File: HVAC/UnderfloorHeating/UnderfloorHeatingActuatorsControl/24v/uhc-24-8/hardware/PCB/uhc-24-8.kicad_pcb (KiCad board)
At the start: 2 copper layers, 118.1 x 69.8 mm, 57 parts, among them J1 WJ126V-5.0-2P, J10 WJ126V-5.0-2P, J11 WJ126V-5.0-2P, J2 ESP-PROG, J3 Conn_02x06_Counter_Clockwise, J4 WJ126V-5.0-2P, J5 WJ126V-5.0-2P, J6 WJ126V-5.0-2P, J7 WJ126V-5.0-2P, J8 WJ126V-5.0-2P, J9 WJ126V-5.0-2P, Q1 2N7002P, Q2 2N7002P, Q3 2N7002P, Q4 2N7002P, Q5 2N7002P, Q6 2N7002P, Q7 2N7002P, Q8 2N7002P, U1 ESP32-WROOM-32D, U2 LM3671MFX-3.3/NOPB

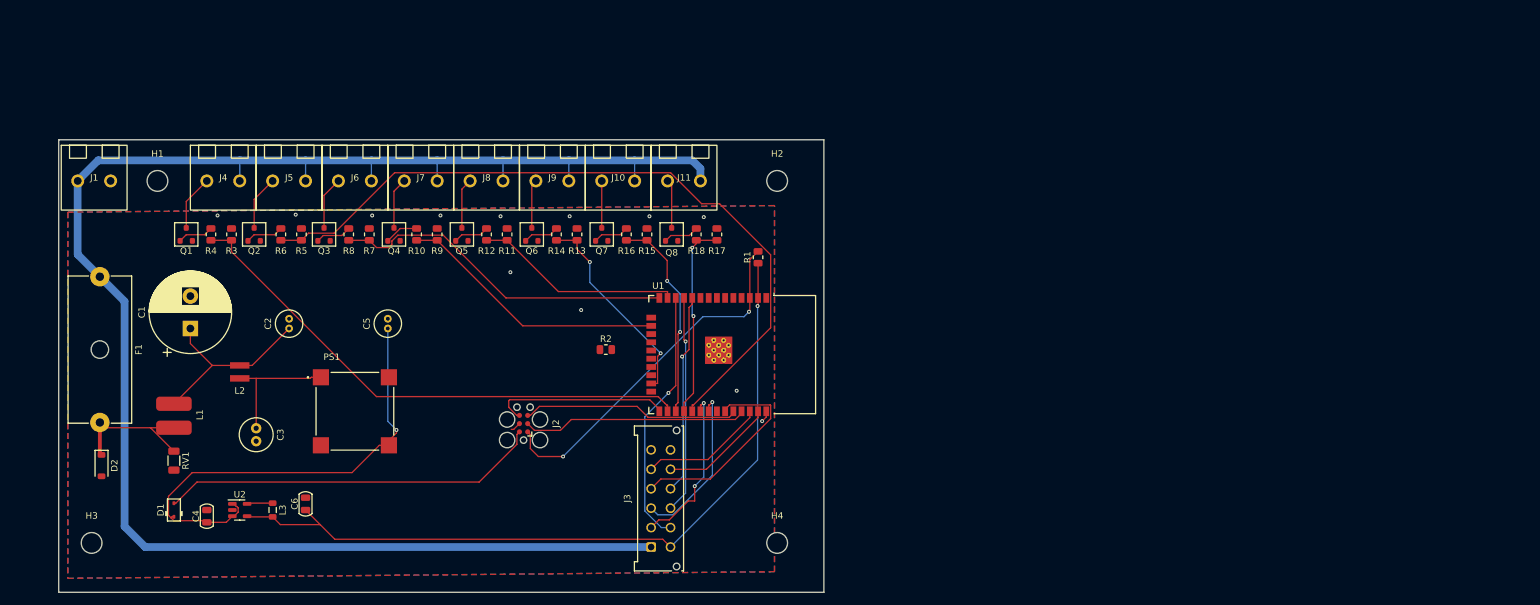
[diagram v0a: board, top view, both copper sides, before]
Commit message: Ready for fabrication
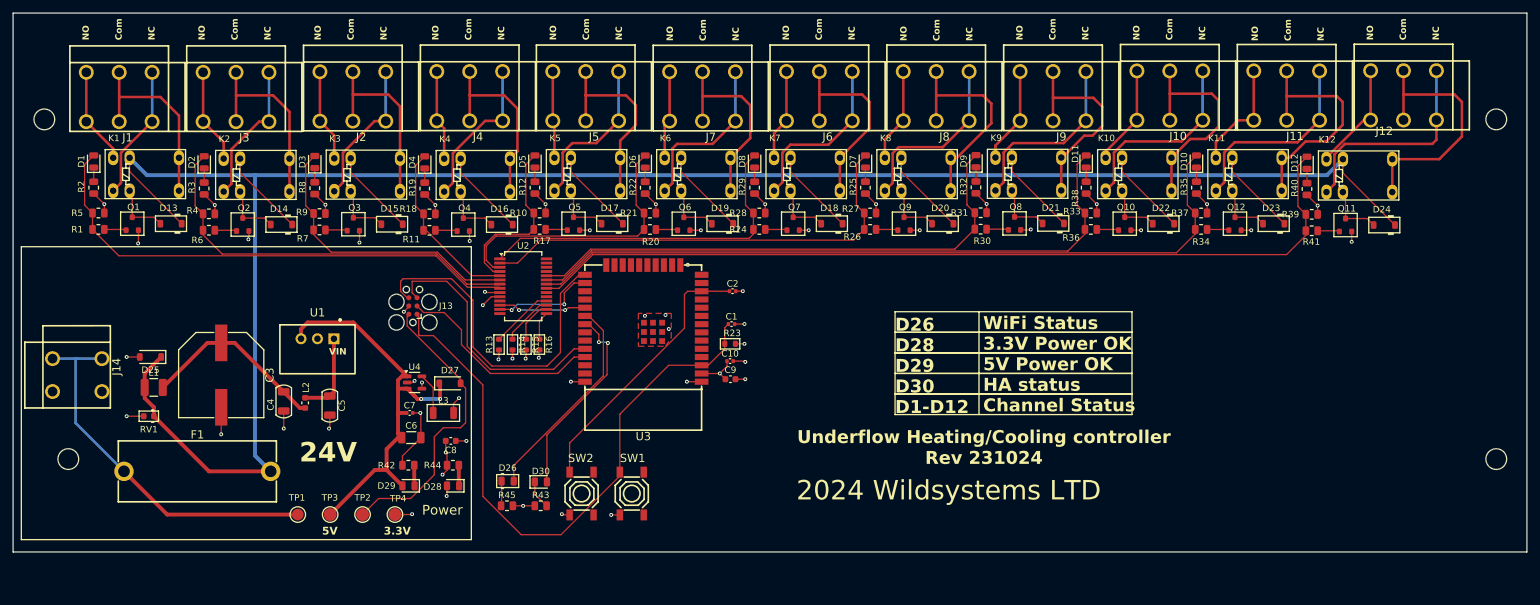
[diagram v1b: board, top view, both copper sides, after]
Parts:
- removed PS1: K7805JT-500R3-LB, K7805JT-500R3:CONV_K7805JT-500R3-LB
- added C10: 0.1uF, Capacitor_SMD:C_0402_1005Metric, F.Cu at (141.7, 91.3)
- added C7: 4.7uF/10V, Capacitor_SMD:C_0402_1005Metric, F.Cu at (92.3, 99.3)
- added C8: 10uF, Capacitor_SMD:C_0603_1608Metric, F.Cu at (98.6, 103.6)
- added C9: 22uF, Capacitor_SMD:C_0603_1608Metric, F.Cu at (141.8, 94.1)
- added D10: KT-0805Y, LED_SMD:LED_0805_2012Metric, F.Cu at (213.7, 60.5)
- added D11: KT-0805Y, LED_SMD:LED_0805_2012Metric, F.Cu at (196.7, 60.5)
- added D12: KT-0805Y, LED_SMD:LED_0805_2012Metric, F.Cu at (230.8, 60.7)
- added D13: 1N4148W, PCM_Diode_SMD_AKL:D_SOD-123, F.Cu at (55.4, 70.1)
- added D14: 1N4148W, PCM_Diode_SMD_AKL:D_SOD-123, F.Cu at (72.5, 70.2)
- added D15: 1N4148W, PCM_Diode_SMD_AKL:D_SOD-123, F.Cu at (89.6, 70.2)
- added D16: 1N4148W, PCM_Diode_SMD_AKL:D_SOD-123, F.Cu at (106.5, 70.2)
- added D17: 1N4148W, PCM_Diode_SMD_AKL:D_SOD-123, F.Cu at (123.5, 70.1)
- added D18: 1N4148W, PCM_Diode_SMD_AKL:D_SOD-123, F.Cu at (157.4, 70.1)
- added D19: 1N4148W, PCM_Diode_SMD_AKL:D_SOD-123, F.Cu at (140.6, 70.1)
- added D20: 1N4148W, PCM_Diode_SMD_AKL:D_SOD-123, F.Cu at (174.6, 70.1)
- added D21: 1N4148W, PCM_Diode_SMD_AKL:D_SOD-123, F.Cu at (191.6, 70.1)
- added D22: 1N4148W, PCM_Diode_SMD_AKL:D_SOD-123, F.Cu at (208.6, 70.1)
- added D23: 1N4148W, PCM_Diode_SMD_AKL:D_SOD-123, F.Cu at (225.6, 70.1)
- added D24: 1N4148W, PCM_Diode_SMD_AKL:D_SOD-123, F.Cu at (242.7, 70.3)
- added D25: BAT46W, Diode_SMD:D_SOD-123, F.Cu at (52.3, 90.7)
- added D26: KT-0805B, Diode_SMD_AKL:D_0805_2012Metric, F.Cu at (107.4, 109.8)
- added D27: 1N5819, Diode_SMD:D_SOD-123, F.Cu at (98.5, 94.7)
- added D28: KT-0805G, LED_SMD:LED_0805_2012Metric, F.Cu at (99.0, 110.6)
- added D29: KT-0805G, LED_SMD:LED_0805_2012Metric, F.Cu at (92.1, 110.6)
- added D3: KT-0805Y, LED_SMD:LED_0805_2012Metric, F.Cu at (77.6, 60.6)
- added D30: KT-0805G, LED_SMD:LED_0805_2012Metric, F.Cu at (112.5, 110.0)
- added D4: KT-0805Y, LED_SMD:LED_0805_2012Metric, F.Cu at (94.6, 60.6)
- added D5: KT-0805Y, LED_SMD:LED_0805_2012Metric, F.Cu at (111.6, 60.5)
- added D6: KT-0805Y, LED_SMD:LED_0805_2012Metric, F.Cu at (128.6, 60.5)
- added D7: KT-0805Y, LED_SMD:LED_0805_2012Metric, F.Cu at (162.6, 60.5)
- added D8: KT-0805Y, LED_SMD:LED_0805_2012Metric, F.Cu at (145.5, 60.5)
- added D9: KT-0805Y, LED_SMD:LED_0805_2012Metric, F.Cu at (179.7, 60.5)
- added J12: WJ126V-5.0-3P, My Footprints:CONN-TH_3P-P5.08_DIBO_DB142V-5.08-3P, F.Cu at (245.7, 50.3)
- added J13: ESP-PROG, Connector:Tag-Connect_TC2030-IDC-FP_2x03_P1.27mm_Vertical, F.Cu at (92.8, 82.8)
- added J14: WJ126V-5.0-2P, My Footprints:CONN-TH_2P-P5.08_DIBO_DB142V-5.08-2P, F.Cu at (41.0, 93.5)
- added K1: BSC-SS-124L, My Footprints:Relay_SPDT_QLRELAY_BSC, F.Cu at (56.7, 59.9)
- added K10: BSC-SS-124L, My Footprints:Relay_SPDT_QLRELAY_BSC, F.Cu at (209.9, 59.9)
- added K11: BSC-SS-124L, My Footprints:Relay_SPDT_QLRELAY_BSC, F.Cu at (226.9, 59.9)
- added K12: BSC-SS-124L, My Footprints:Relay_SPDT_QLRELAY_BSC, F.Cu at (244.0, 60.1)
- added K2: BSC-SS-124L, My Footprints:Relay_SPDT_QLRELAY_BSC, F.Cu at (73.7, 60.1)
- added K3: BSC-SS-124L, My Footprints:Relay_SPDT_QLRELAY_BSC, F.Cu at (90.8, 60.0)
- added K4: BSC-SS-124L, My Footprints:Relay_SPDT_QLRELAY_BSC, F.Cu at (107.8, 60.1)
- added K5: BSC-SS-124L, My Footprints:Relay_SPDT_QLRELAY_BSC, F.Cu at (124.8, 59.9)
- added K6: BSC-SS-124L, My Footprints:Relay_SPDT_QLRELAY_BSC, F.Cu at (141.8, 59.9)
- added K7: BSC-SS-124L, My Footprints:Relay_SPDT_QLRELAY_BSC, F.Cu at (158.7, 59.9)
- added K8: BSC-SS-124L, My Footprints:Relay_SPDT_QLRELAY_BSC, F.Cu at (175.8, 59.9)
- added K9: BSC-SS-124L, My Footprints:Relay_SPDT_QLRELAY_BSC, F.Cu at (192.9, 59.9)
- added Q10: 2N7002P, Package_TO_SOT_SMD_AKL:SOT-23, F.Cu at (202.7, 70.1)
- added Q11: 2N7002P, Package_TO_SOT_SMD_AKL:SOT-23, F.Cu at (236.7, 70.3)
- added Q12: 2N7002P, Package_TO_SOT_SMD_AKL:SOT-23, F.Cu at (219.7, 70.1)
- added Q9: 2N7002P, Package_TO_SOT_SMD_AKL:SOT-23, F.Cu at (168.6, 70.1)
- added R19: 56R, Resistor_SMD:R_0805_2012Metric, F.Cu at (94.6, 64.7)
- added R20: 510R, Resistor_SMD:R_0805_2012Metric, F.Cu at (129.4, 71.0)
- added R21: 4.7k, Resistor_SMD:R_0805_2012Metric, F.Cu at (129.4, 68.5)
- added R22: 56R, Resistor_SMD:R_0805_2012Metric, F.Cu at (128.6, 64.5)
- added R23: 10K, PCM_Resistor_SMD_AKL:R_0603_1608Metric, F.Cu at (141.7, 88.6)
- added R24: 510R, Resistor_SMD:R_0805_2012Metric, F.Cu at (146.2, 71.0)
- added R25: 56R, Resistor_SMD:R_0805_2012Metric, F.Cu at (162.6, 64.5)
- added R26: 510R, Resistor_SMD:R_0805_2012Metric, F.Cu at (163.4, 71.0)
- added R27: 4.7k, Resistor_SMD:R_0805_2012Metric, F.Cu at (163.4, 68.5)
- added R28: 4.7k, Resistor_SMD:R_0805_2012Metric, F.Cu at (146.2, 68.5)
- added R29: 56R, Resistor_SMD:R_0805_2012Metric, F.Cu at (145.5, 64.5)
- added R30: 510R, Resistor_SMD:R_0805_2012Metric, F.Cu at (180.4, 70.9)
- added R31: 4.7k, Resistor_SMD:R_0805_2012Metric, F.Cu at (180.4, 68.4)
- added R32: 56R, Resistor_SMD:R_0805_2012Metric, F.Cu at (179.7, 64.5)
- added R33: 4.7k, Resistor_SMD:R_0805_2012Metric, F.Cu at (197.4, 68.5)
- added R34: 510R, Resistor_SMD:R_0805_2012Metric, F.Cu at (214.4, 71.0)
- added R35: 56R, Resistor_SMD:R_0805_2012Metric, F.Cu at (213.7, 64.5)
- added R36: 510R, Resistor_SMD:R_0805_2012Metric, F.Cu at (197.4, 71.0)
- added R37: 4.7k, Resistor_SMD:R_0805_2012Metric, F.Cu at (214.4, 68.5)
- added R38: 56R, Resistor_SMD:R_0805_2012Metric, F.Cu at (196.7, 64.5)
- added R39: 4.7k, Resistor_SMD:R_0805_2012Metric, F.Cu at (231.5, 68.7)
- added R40: 56R, Resistor_SMD:R_0805_2012Metric, F.Cu at (230.8, 64.7)
- added R41: 510R, Resistor_SMD:R_0805_2012Metric, F.Cu at (231.5, 71.2)
- added R42: 20R, Resistor_SMD:R_0805_2012Metric, F.Cu at (92.1, 107.4)
- added R43: 20R, Resistor_SMD:R_0805_2012Metric, F.Cu at (112.5, 113.6)
- added R44: 20R, Resistor_SMD:R_0805_2012Metric, F.Cu at (98.9, 107.4)
- added R45: 15R, Resistor_SMD:R_0805_2012Metric, F.Cu at (107.3, 113.6)
- added SW1: Reboot, My Footprints:SW-SMD_4P-L5.1-W5.1-P3.70-LS6.5-TL-2, F.Cu at (126.6, 111.8)
- added SW2: Clear, My Footprints:SW-SMD_4P-L5.1-W5.1-P3.70-LS6.5-TL-2, F.Cu at (118.8, 111.8)
- added TP1: 24V, TestPoint:TestPoint_Pad_D2.0mm, F.Cu at (75.0, 115.0)
- added TP2: 5V_USB, TestPoint:TestPoint_Pad_D2.0mm, F.Cu at (85.0, 115.0)
- added TP3: 5V, TestPoint:TestPoint_Pad_D2.0mm, F.Cu at (80.0, 115.0)
- added TP4: 3.3V, TestPoint:TestPoint_Pad_D2.0mm, F.Cu at (90.0, 115.0)
- added U3: ESP32-WROOM-32D, My Footprints:WIFI-SMD_ESP32-WROOM-32E-A, F.Cu at (128.3, 85.5)
- added U4: LM3671MFX-3.3/NOPB, Package_TO_SOT_SMD:TSOT-23-5, F.Cu at (93.0, 94.6)
- C1: value 680uF/50V -> 1uF; footprint Capacitor_THT:CP_Radial_D12.5mm_P5.00mm -> Capacitor_SMD:C_0402_1005Metric
- C2: value 4.7uF/50V -> 0.1uF; footprint Capacitor_THT_AKL:C_Radial_D4.0mm_H5.0mm_P1.50mm -> Capacitor_SMD:C_0402_1005Metric
- C3: value 10uF/50V -> 680uF/50V; footprint Capacitor_THT:C_Radial_D5.0mm_H11.0mm_P2.00mm -> My Footprints:CAP-SMD_BD12.5-L13.0-W13.0-LS14.4-FD
- C4: value 4.7uF -> 4.7uF/63V; footprint Capacitor_SMD_AKL:C_0805_2012Metric -> Capacitor_SMD_AKL:C_1206_3216Metric
- C5: value 22uF/10V -> 10uF/50V; footprint Capacitor_THT:C_Radial_D4.0mm_H7.0mm_P1.50mm -> Capacitor_SMD_AKL:C_1206_3216Metric
- C6: value 10uF -> 22uF/10V; footprint Capacitor_SMD_AKL:C_0805_2012Metric -> Capacitor_SMD:C_1206_3216Metric
- D1: value 1N5819 -> KT-0805Y; footprint Diode_SMD_AKL:D_SOD-323 -> LED_SMD:LED_0805_2012Metric
- D2: value BAT46W -> KT-0805Y; footprint Diode_SMD:D_SOD-123 -> LED_SMD:LED_0805_2012Metric
- F1: value C3131 -> Fuse; footprint Fuse:Fuseholder_Cylinder-5x20mm_Schurter_0031_8201_Horizontal_Open -> My Footprints:FUSE-TH_L24.4-W9.4-P22.60
- J1, J10, J11, J4, J5, J6, J7, J8, J9: value WJ126V-5.0-2P -> WJ126V-5.0-3P; footprint My Footprints:WJ500V-5.08-2P -> My Footprints:CONN-TH_3P-P5.08_DIBO_DB142V-5.08-3P
- J2: value ESP-PROG -> WJ126V-5.0-3P; footprint Connector:Tag-Connect_TC2030-IDC-FP_2x03_P1.27mm_Vertical -> My Footprints:CONN-TH_3P-P5.08_DIBO_DB142V-5.08-3P
- J3: value Conn_02x06_Counter_Clockwise -> WJ126V-5.0-3P; footprint Connector_Molex:Molex_Micro-Fit_3.0_43045-1212_2x06_P3.00mm_Vertical -> My Footprints:CONN-TH_3P-P5.08_DIBO_DB142V-5.08-3P
- L1: value BC54-820M(CD) -> FHW1210IF820JST; footprint My Footprints:BC54-820M -> Inductor_SMD:L_1210_3225Metric
- L2: value CD31 220M -> 22uH; footprint My Footprints:CD31 -> Inductor_SMD:L_0603_1608Metric
- L3: footprint Inductor_SMD:L_0805_2012Metric -> Ferrite_SMD_AKL:Ferrite_1206_3216Metric
- R1: value 4.7K -> 510R
- R10, R18, R4: value 510R -> 4.7k
- R11, R17, R7: value 4.7k -> 510R
- R12, R8: value 510R -> 56R
- R13, R15: value 4.7k -> 10K; footprint Resistor_SMD:R_0805_2012Metric -> PCM_Resistor_SMD_AKL:R_0603_1608Metric
- R14, R16: value 510R -> 10K; footprint Resistor_SMD:R_0805_2012Metric -> PCM_Resistor_SMD_AKL:R_0603_1608Metric
- R2, R3: value 4.7k -> 56R
- RV1: value SFI1206SV471-201A -> RL0603E024M250K; footprint Resistor_SMD:R_1206_3216Metric -> Diode_SMD_AKL:D_0603_1608Metric
- U1: value ESP32-WROOM-32D -> K7805-500R3; footprint My Footprints:ESP32-WROOM-32-0.3-via -> My Footprints:PWRM-TH_K78XX-500R3
- U2: value LM3671MFX-3.3/NOPB -> MCP23017_SS; footprint Package_TO_SOT_SMD:TSOT-23-5 -> Package_SO:SSOP-28_5.3x10.2mm_P0.65mm
- moved H4 111.8 mm to (260.0, 106.4)
- moved H2 111.4 mm to (260.0, 54.0)
- moved R1 101.9 mm to (44.2, 71.0), turned to 0 degrees
- moved J3 94.5 mm to (65.5, 50.5), turned to 180 degrees
- moved J11 94.0 mm to (227.6, 50.3), turned to 180 degrees
- moved J10 86.2 mm to (209.6, 50.3), turned to 180 degrees
- moved C1 83.5 mm to (142.0, 85.6), turned to 0 degrees
- moved R2 82.9 mm to (43.5, 64.5), turned to 90 degrees
- moved J9 78.4 mm to (191.6, 50.4), turned to 180 degrees
- moved J6 72.9 mm to (155.5, 50.4), turned to 180 degrees
- moved J8 70.6 mm to (173.5, 50.4), turned to 180 degrees
- moved C2 68.7 mm to (142.1, 80.5), turned to 0 degrees
- moved U1 61.1 mm to (78.0, 87.9), turned to 0 degrees
- moved J2 57.0 mm to (83.5, 50.5), turned to 180 degrees
- moved U2 55.7 mm to (109.8, 79.8)
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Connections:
- C1 pad 1: Net-(C1-Pad1) -> /EN
- C2 pad 1: Net-(C1-Pad1) -> /IO27
- C3 pad 1: Net-(PS1-+VIN) -> Net-(C3-Pad1)
- C4 pad 1: Net-(D1-K) -> Net-(C3-Pad1)
- C5 pad 1: Net-(D1-K) -> Net-(U1-IN)
- C6 pad 1: /Power/+3V3 -> +5V
- D1 pad 2: /5V_USB -> /Out1/IN
- D2 pad 2: GND -> /Out2/IN
- F1 pad 2: Net-(D2-K) -> +24V_FUSED
- J1 pad 1: +24V -> /Out1/NC
- J1 pad 2: GND -> /Out1/COM
- J10 pad 1: Net-(J10-Pin_1) -> /Out10/NC
- J10 pad 2: +24V -> /Out10/COM
- J11 pad 1: Net-(J11-Pin_1) -> /Out11/NC
- J11 pad 2: +24V -> /Out11/COM
- J2 pad 1: /EN -> /Out3/NC
- J2 pad 2: /5V_USB -> /Out3/COM
- J2 pad 3: /GPIO01 -> /Out3/NO
- J3 pad 1: +24V -> /Out2/NC
- J3 pad 2: /IO16 -> /Out2/COM
- J3 pad 3: /IO17 -> /Out2/NO
- J4 pad 1: Net-(J4-Pin_1) -> /Out4/NC
- J4 pad 2: +24V -> /Out4/COM
- J5 pad 1: Net-(J5-Pin_1) -> /Out5/NC
- J5 pad 2: +24V -> /Out5/COM
- J6 pad 1: Net-(J6-Pin_1) -> /Out7/NC
- J6 pad 2: +24V -> /Out7/COM
- J7 pad 1: Net-(J7-Pin_1) -> /Out6/NC
- J7 pad 2: +24V -> /Out6/COM
- J8 pad 1: Net-(J8-Pin_1) -> /Out8/NC
- J8 pad 2: +24V -> /Out8/COM
- J9 pad 1: Net-(J9-Pin_1) -> /Out9/NC
- J9 pad 2: +24V -> /Out9/COM
- L1 pad 1: Net-(D2-K) -> +24V_FUSED
- L1 pad 2: Net-(C1-Pad1) -> Net-(C3-Pad1)
- L2 pad 1: Net-(C1-Pad1) -> Net-(C3-Pad1)
- L2 pad 2: Net-(PS1-+VIN) -> Net-(U1-IN)
- L3 pad 1: Net-(U2-SW) -> Net-(U4-SW)
- L3 pad 2: /Power/+3V3 -> /3v3
- Q1 pad 3: Net-(J4-Pin_1) -> Net-(D13-A)
- Q2 pad 3: Net-(J5-Pin_1) -> Net-(D14-A)
- Q3 pad 3: Net-(J6-Pin_1) -> Net-(D15-A)
- Q4 pad 3: Net-(J7-Pin_1) -> Net-(D16-A)
- Q5 pad 3: Net-(J8-Pin_1) -> Net-(D17-A)
- Q6 pad 3: Net-(J9-Pin_1) -> Net-(D19-A)
- Q7 pad 3: Net-(J10-Pin_1) -> Net-(D18-A)
- Q8 pad 3: Net-(J11-Pin_1) -> Net-(D21-A)
- R1 pad 1: /Power/+3V3 -> /Out1/IN
- R1 pad 2: /EN -> Net-(Q1-G)
- R10 pad 1: /Out4/IN -> GND
- R10 pad 2: Net-(Q4-G) -> /Out5/IN
- R11 pad 1: GND -> /Out4/IN
- R11 pad 2: /Out5/IN -> Net-(Q4-G)
- R12 pad 1: /Out5/IN -> GND
- R12 pad 2: Net-(Q5-G) -> Net-(D5-K)
- R13 pad 1: GND -> /3v3
- R13 pad 2: /Out6/IN -> Net-(U2-~{RESET})
- R14 pad 1: /Out6/IN -> Net-(U2-A2)
- R14 pad 2: Net-(Q6-G) -> GND
- R15 pad 1: GND -> Net-(U2-A1)
- R15 pad 2: /Out7/IN -> GND
- R16 pad 1: /Out7/IN -> Net-(U2-A0)
- R16 pad 2: Net-(Q7-G) -> GND
- R17 pad 1: GND -> /Out5/IN
- R17 pad 2: /Out8/IN -> Net-(Q5-G)
- R18 pad 1: /Out8/IN -> GND
- R18 pad 2: Net-(Q8-G) -> /Out4/IN
- R2 pad 2: Net-(U1-IO26) -> Net-(D1-K)
- R3 pad 2: /Out1/IN -> Net-(D2-K)
- R4 pad 1: /Out1/IN -> GND
- R4 pad 2: Net-(Q1-G) -> /Out2/IN
- R5 pad 2: /Out2/IN -> /Out1/IN
- R7 pad 1: GND -> /Out3/IN
- R7 pad 2: /Out3/IN -> Net-(Q3-G)
- R8 pad 1: /Out3/IN -> GND
- R8 pad 2: Net-(Q3-G) -> Net-(D3-K)
- R9 pad 2: /Out4/IN -> /Out3/IN
- RV1 pad 1: Net-(D2-K) -> +24V_FUSED
- U1 pad 1: GND -> Net-(U1-IN)
- U1 pad 2: /Power/+3V3 -> GND
- U1 pad 3: /EN -> +5V
- U2 pad 1: Net-(D1-K) -> /Out7/IN
- U2 pad 2: GND -> /Out8/IN
- U2 pad 3: Net-(D1-K) -> /Out6/IN
- U2 pad 4: /Power/+3V3 -> /Out5/IN
- U2 pad 5: Net-(U2-SW) -> /Out4/IN
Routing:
- net +24V_FUSED: track 0.00 -> 457.5 mm
- net +24V: track 261.0 -> 57.7 mm
- net /Out12/IN: track 0.00 -> 133.8 mm
- net /Power/+3V3: track 119.9 -> 0.00 mm, vias 1 -> 0
- net GND: track 3.43 -> 120.4 mm, vias 12 -> 51
- net /Out11/IN: track 0.00 -> 116.6 mm
- net /Out10/IN: track 0.00 -> 99.3 mm
- net /Out9/IN: track 0.00 -> 81.6 mm
- net Net-(D1-K): track 73.8 -> 2.19 mm, vias 1 -> 0
- net +5V: track 0.00 -> 64.9 mm, vias 0 -> 2
- net /BOOT: track 0.00 -> 52.9 mm
- net /Out2/IN: track 114.5 -> 62.2 mm
- net /IO27: track 0.00 -> 41.8 mm
- net /RXD0: track 0.00 -> 40.5 mm
- net /Out8/IN: track 30.5 -> 70.9 mm, vias 2 -> 0
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- added copper zone on In1.Cu, net /3v3
- added copper zone on In2.Cu, net GND
- removed copper zone on B.Cu, net GND
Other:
- board size 118.1 x 69.8 mm -> 233.7 x 83.2 mm
- copper layers 2 -> 4
- board text added: "2024 Wildsystems LTD"
- board text added: "24V"
- board text added: "3.3V"
- board text added: "3.3V Power OK"
- board text added: "5V"
- board text added: "5V Power OK"
- board text added: "Channel Status"
- board text added: "Com"
- board text added: "D1-D12"
- board text added: "D26"
- board text added: "D28"
- board text added: "D29"
- board text added: "D30"
- board text added: "HA status"
- board text added: "NC"
- board text added: "NO"
- board text added: "Power"
- board text added: "Underflow Heating/Cooling controller Rev 231024"
- board text added: "WiFi Status"
